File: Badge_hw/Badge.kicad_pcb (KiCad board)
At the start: 2 copper layers, 114 x 62 mm, 147 parts, among them Q1 IRLML9303, Q2 BC848

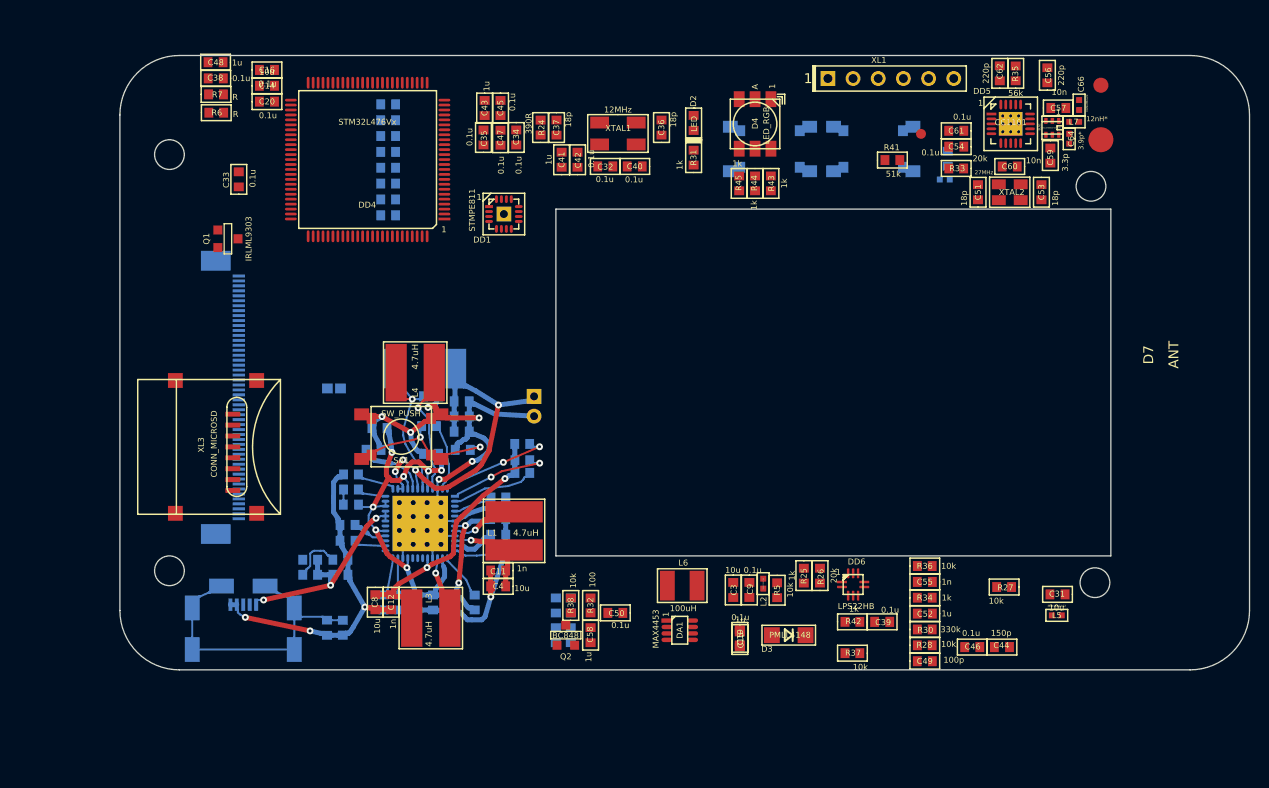
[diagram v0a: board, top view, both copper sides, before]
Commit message: pcb full 1.0
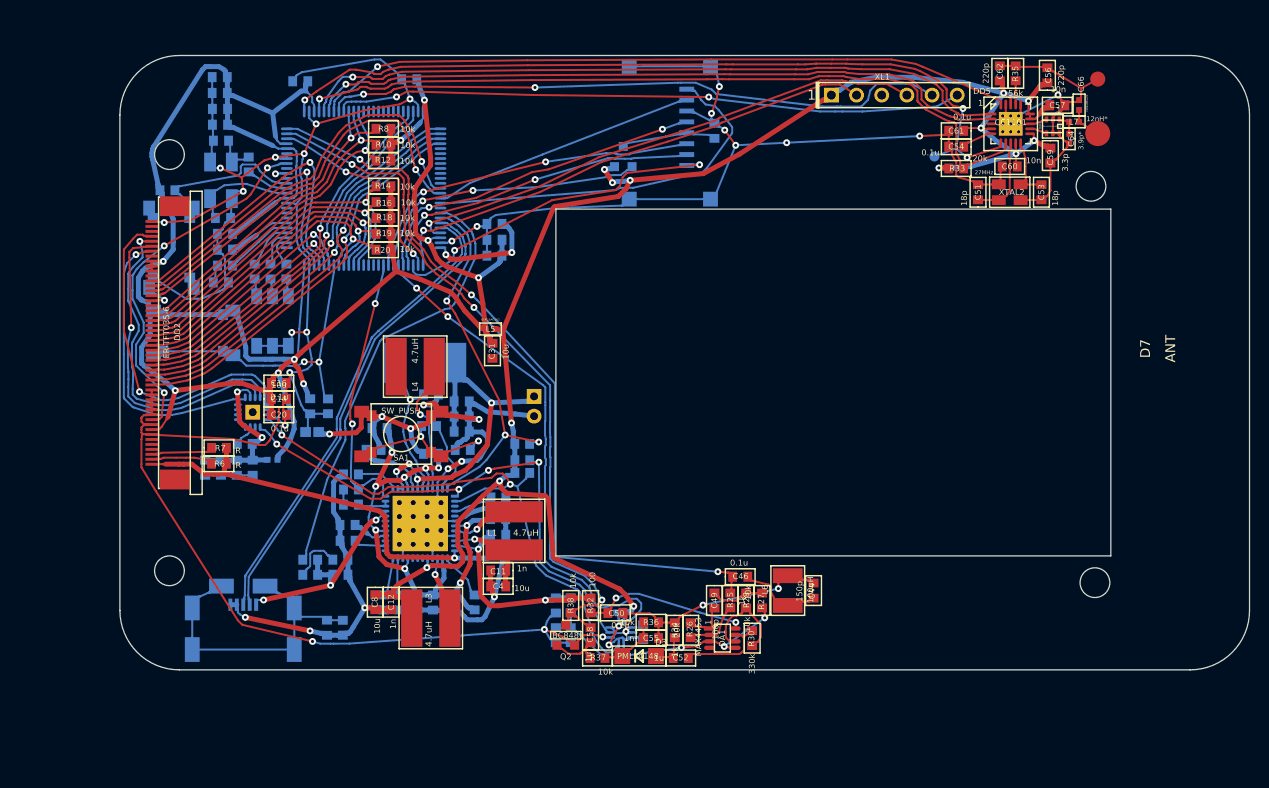
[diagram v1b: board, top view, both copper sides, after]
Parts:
- C15, C19, C3, C32, C33, C34, C35, C36, C37, C38, C39, C40, C41, C42, C43, C45, C47, C48, C9, D2, D4, DD1, DD4, DD6, L2, Q1, R24, R31, R41, R42, R43, R44, R45, R5, TP1, XL3, XTAL1: moved to B.Cu
- DD2, R10, R12, R14, R16, R18, R19, R20, R8: moved to F.Cu
- moved R41 73.2 mm to (104.8, 63.6), turned to 180 degrees
- moved SA2 71.5 mm to (105.2, 69.4), turned to 270 degrees
- moved L5 64.0 mm to (137.4, 77.6)
- moved C31 62.1 mm to (137.6, 79.8), turned to 270 degrees
- moved C39 61.7 mm to (119.2, 85.4), turned to 270 degrees
- moved SA3 61.1 mm to (107.4, 78.0)
- moved R42 57.2 mm to (121.0, 85.4), turned to 90 degrees
- moved C68 56.8 mm to (152.8, 108.2)
- moved C15 56.7 mm to (108.6, 91.6)
- moved R5 55.7 mm to (112.6, 89.2), turned to 0 degrees
- moved XL3 55.7 mm to (154.8, 57.8)
- moved C19 55.1 mm to (110.2, 91.6)
- moved L8 54.5 mm to (150.6, 106.2), turned to 0 degrees
- moved C9 53.2 mm to (111.8, 91.6)
- moved D4 52.6 mm to (115.4, 76.8), turned to 90 degrees
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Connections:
- C15 pad 2: Net-(C15-Pad2) -> GNDS
- C19 pad 2: Net-(C15-Pad2) -> GNDS
- C3 pad 2: Net-(C15-Pad2) -> GNDS
- C9 pad 2: Net-(C15-Pad2) -> GNDS
- DD2 pad 43: GNDA -> GNDS
- DD2 pad 48: GNDA -> GNDS
- DD2 pad 49: GNDA -> GNDS
- DD2 pad 50: GNDA -> GNDS
- DD4 pad 15: /SCK -> /SCL
- DD4 pad 67: /CHARGING -> Net-(DD4-Pad67)
- XL1 pad 3: GNDA -> GNDS
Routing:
- net +3V3: track 27.9 -> 422.7 mm, vias 2 -> 24
- net GNDS: track 0.00 -> 387.4 mm, vias 0 -> 27
- net /CC_GDO0: track 0.00 -> 82.6 mm, vias 0 -> 3
- net /CC_CS: track 0.00 -> 78.1 mm, vias 0 -> 1
- net /klNFC_Tx: track 0.00 -> 78.0 mm, vias 0 -> 3
- net /CC_SCK: track 0.00 -> 72.0 mm, vias 0 -> 1
- net /klNFC_Rx: track 0.00 -> 71.9 mm, vias 0 -> 3
- net /CC_MISO: track 0.00 -> 71.0 mm, vias 0 -> 1
- net /CC_MOSI: track 0.00 -> 70.9 mm, vias 0 -> 1
- net /UART_RX: track 0.00 -> 63.3 mm, vias 0 -> 2
- net /UART_TX: track 0.00 -> 63.1 mm, vias 0 -> 2
- net /SWD_IO: track 0.00 -> 53.0 mm, vias 0 -> 1
- net /PRESSURE_INT: track 0.00 -> 52.2 mm, vias 0 -> 2
- net /SWD_CLK: track 0.00 -> 50.3 mm, vias 0 -> 1
- net /SCL: track 8.38 -> 58.6 mm, vias 0 -> 2
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
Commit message: *pcb 2.0
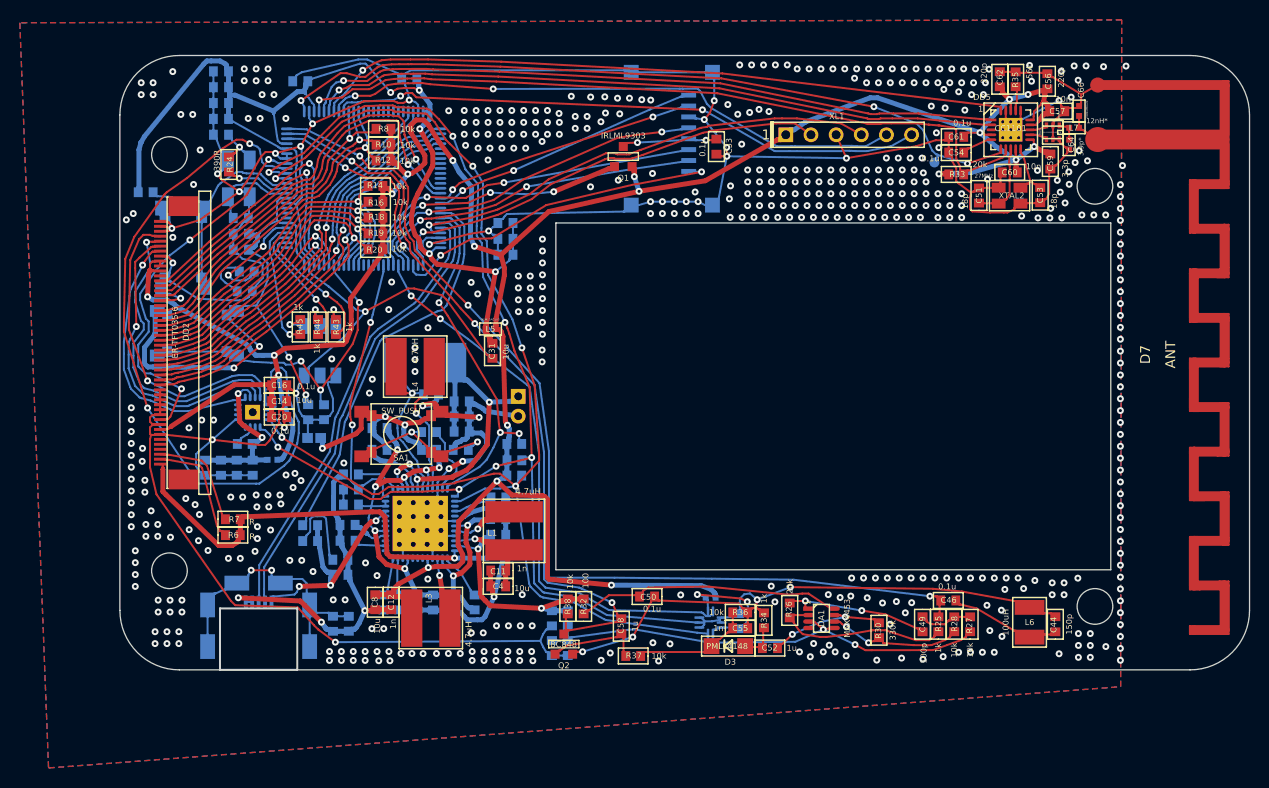
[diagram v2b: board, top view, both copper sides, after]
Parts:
- added G***: LOGO, Badge_hw:logo, B.Cu at (207.8, 80.7)
- C33, Q1, R24, R43, R44, R45: moved to F.Cu
- moved C44 24.6 mm to (194.4, 107.4)
- moved L6 24.6 mm to (191.8, 107.2)
- moved C46 21.1 mm to (183.6, 105.0)
- moved C49 21.1 mm to (181.0, 107.4)
- moved R25 21.1 mm to (182.6, 107.4)
- moved R27 21.1 mm to (185.8, 107.4)
- moved R28 21.1 mm to (184.2, 107.4)
- moved R30 12.8 mm to (176.6, 108.0)
- moved DA1 10.2 mm to (170.8, 106.8)
- moved R26 10.2 mm to (167.6, 106.0)
- moved C68 9.73 mm to (162.5, 107.1)
- moved L8 9.14 mm to (159.6, 104.7)
- moved C52 9.06 mm to (165.6, 109.8)
- moved C55 9.06 mm to (162.6, 107.8)
- moved D3 9.06 mm to (161.4, 109.6)
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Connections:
- C31 pad 1: +3V3 -> MCU_PWR
- C32 pad 1: +3V3 -> MCU_PWR
- C34 pad 1: +3V3 -> MCU_PWR
- C35 pad 1: +3V3 -> MCU_PWR
- C38 pad 1: +3V3 -> MCU_PWR
- C39 pad 1: +3V3 -> MCU_PWR
- C40 pad 1: +3V3 -> MCU_PWR
- C41 pad 1: +3V3 -> MCU_PWR
- C42 pad 1: +3V3 -> MCU_PWR
- C43 pad 1: +3V3 -> MCU_PWR
- C45 pad 1: +3V3 -> MCU_PWR
- C47 pad 1: +3V3 -> MCU_PWR
- C48 pad 1: +3V3 -> MCU_PWR
- DD4 pad 100: +3V3 -> MCU_PWR
- DD4 pad 11: +3V3 -> MCU_PWR
- DD4 pad 21: +3V3 -> MCU_PWR
- DD4 pad 22: +3V3 -> MCU_PWR
- DD4 pad 28: +3V3 -> MCU_PWR
- DD4 pad 50: +3V3 -> MCU_PWR
- DD4 pad 6: +3V3 -> MCU_PWR
- DD4 pad 73: +3V3 -> MCU_PWR
- DD4 pad 75: +3V3 -> MCU_PWR
- L5 pad 1: +3V3 -> MCU_PWR
- R41 pad 2: +3V3 -> MCU_PWR
- SA3 pad 2: +3V3 -> MCU_PWR
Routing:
- net MCU_PWR: track 0.00 -> 178.0 mm, vias 0 -> 9
- net +3V3: track 422.7 -> 297.0 mm, vias 24 -> 19
- net GNDS: track 387.4 -> 495.3 mm, vias 27 -> 31
- net /TOUCH_INT: track 0.00 -> 73.7 mm, vias 0 -> 2
- net /SCL: track 58.6 -> 126.0 mm, vias 2 -> 5
- net /SDA: track 55.1 -> 121.5 mm, vias 5 -> 7
- net /klNFC_Tx: track 78.0 -> 100.6 mm
- net VGND: track 27.2 -> 48.2 mm, vias 3 -> 2
- net Net-(DA1-Pad2): track 5.84 -> 18.4 mm
- net /SD_DAT1: track 38.6 -> 27.5 mm, vias 0 -> 2
- net Net-(C49-Pad2): track 4.35 -> 15.0 mm, vias 0 -> 2
- net Net-(C50-Pad2): track 16.7 -> 26.9 mm, vias 2 -> 0
- net Net-(DD4-Pad2): track 3.33 -> 13.4 mm, vias 0 -> 1
- net Net-(DD4-Pad3): track 3.86 -> 13.2 mm, vias 0 -> 1
- net Net-(DD4-Pad4): track 5.02 -> 13.0 mm, vias 0 -> 1
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- added copper zone on B.Cu, net GNDS
- added copper zone on F.Cu, net GNDS
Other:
- outline, holes or cut-outs redrawn
- rule via_min_size: 0.4 -> 0.7

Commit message: Working FW project
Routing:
- net GNDS: vias 31 -> 539
- net (no net): vias 508 -> 0
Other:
- rule pad_to_mask_clearance: 0.2 -> 0.1
